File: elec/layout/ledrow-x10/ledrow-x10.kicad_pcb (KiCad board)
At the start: 2 copper layers, 20 parts

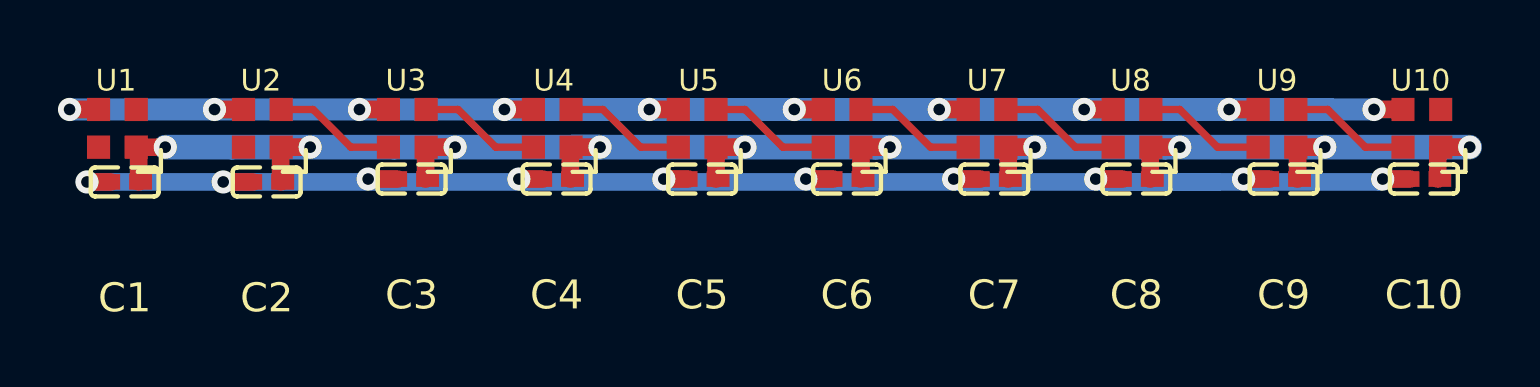
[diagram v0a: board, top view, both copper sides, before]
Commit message: fixing
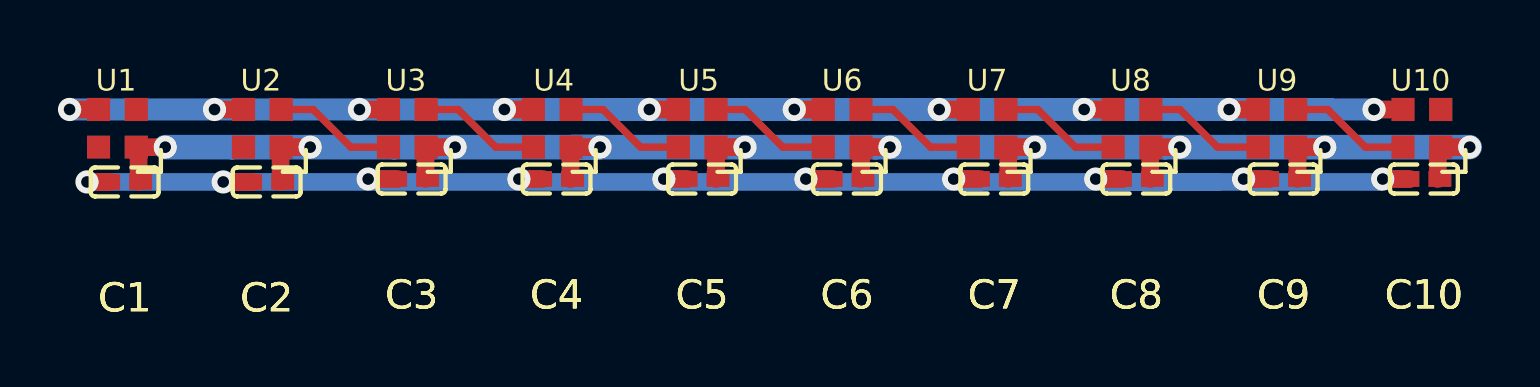
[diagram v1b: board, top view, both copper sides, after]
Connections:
- net vcc-4 renamed io-4
- U1 pad 2: vcc-2 -> io
- U10 pad 4: io -> vcc
- U2 pad 2: io-1 -> io-2
- U2 pad 4: vcc-2 -> io
- U3 pad 2: io-2 -> io-5
- U3 pad 4: io-1 -> io-2
- U4 pad 2: vcc-1 -> io-3
- U4 pad 4: io-2 -> io-5
- U5 pad 4: vcc-1 -> io-3
- U6 pad 2: vcc -> io-6
- U7 pad 2: vcc-3 -> io-1
- U7 pad 4: vcc -> io-6
- U8 pad 2: io-3 -> vcc-1
- U8 pad 4: vcc-3 -> io-1
- U9 pad 2: io -> vcc
- U9 pad 4: io-3 -> vcc-1
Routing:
- net vcc-3: track 4.24 -> 0.00 mm
- net io-6: track 0.00 -> 4.24 mm
- net io-5: track 0.00 -> 4.24 mm
- net io: track 4.24 -> 0.00 mm

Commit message: build with v3
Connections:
- U1 pad 2: io -> io-4
- U10 pad 4: vcc -> io-2
- U2 pad 2: io-2 -> io
- U2 pad 4: io -> io-4
- U3 pad 2: io-5 -> vcc
- U3 pad 4: io-2 -> io
- U4 pad 2: io-3 -> vcc-2
- U4 pad 4: io-5 -> vcc
- U5 pad 2: io-4 -> io-3
- U5 pad 4: io-3 -> vcc-2
- U6 pad 2: io-6 -> io-1
- U6 pad 4: io-4 -> io-3
- U7 pad 2: io-1 -> vcc-1
- U7 pad 4: io-6 -> io-1
- U8 pad 2: vcc-1 -> vcc-3
- U8 pad 4: io-1 -> vcc-1
- U9 pad 2: vcc -> io-2
- U9 pad 4: vcc-1 -> vcc-3
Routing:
- net vcc-2: track 0.00 -> 4.24 mm
- net io-6: track 4.24 -> 0.00 mm
- net io-5: track 4.24 -> 0.00 mm
- net io: track 0.00 -> 4.24 mm
- net vcc-3: track 0.00 -> 4.24 mm
- net io-4: track 4.24 -> 0.00 mm
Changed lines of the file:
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@@
     (net 1 "hv")
     (net 2 "gnd")
-    (net 3 "io-2")
-    (net 4 "io")
-    (net 5 "io-5")
-    (net 6 "io-3")
-    (net 7 "io-4")
-    (net 8 "io-6")
-    (net 9 "io-1")
-    (net 10 "vcc-1")
-    (net 11 "vcc")
+    (net 3 "io")
+    (net 4 "io-4")
+    (net 5 "vcc")
+    (net 6 "vcc-2")
+    (net 7 "io-3")
+    (net 8 "io-1")
+    (net 9 "vcc-1")
+    (net 10 "vcc-3")
+    (net 11 "io-2")
     (net 12 "DOUT")
     (net 13 "DIN")
@@
             (size 0.8 0.8)
             (layers "F.Cu" "F.Mask" "F.Paste")
-            (net 11 "vcc")
+            (net 11 "io-2")
             (pintype "stereo")
         )
@@
             (size 0.8 0.8)
             (layers "F.Cu" "F.Mask" "F.Paste")
-            (net 10 "vcc-1")
+            (net 10 "vcc-3")
             (pintype "stereo")
         )
@@
             (size 0.8 0.8)
             (layers "F.Cu" "F.Mask" "F.Paste")
-            (net 3 "io-2")
+            (net 3 "io")
             (pintype "stereo")
         )
@@
             (size 0.8 0.8)
             (layers "F.Cu" "F.Mask" "F.Paste")
-            (net 4 "io")
+            (net 4 "io-4")
             (pintype "stereo")
         )
@@
             (size 0.8 0.8)
             (layers "F.Cu" "F.Mask" "F.Paste")
-            (net 4 "io")
+            (net 4 "io-4")
             (pintype "stereo")
         )
@@
             (size 0.8 0.8)
             (layers "F.Cu" "F.Mask" "F.Paste")
-            (net 9 "io-1")
+            (net 9 "vcc-1")
             (pintype "stereo")
         )
@@
             (size 0.8 0.8)
             (layers "F.Cu" "F.Mask" "F.Paste")
-            (net 8 "io-6")
+            (net 8 "io-1")
             (pintype "stereo")
         )
@@
             (size 0.8 0.8)
             (layers "F.Cu" "F.Mask" "F.Paste")
-            (net 7 "io-4")
+            (net 7 "io-3")
             (pintype "stereo")
         )
@@
             (size 0.8 0.8)
             (layers "F.Cu" "F.Mask" "F.Paste")
-            (net 6 "io-3")
+            (net 6 "vcc-2")
             (pintype "stereo")
         )
@@
             (size 0.8 0.8)
             (layers "F.Cu" "F.Mask" "F.Paste")
-            (net 11 "vcc")
+            (net 11 "io-2")
             (pintype "stereo")
         )
@@
             (size 0.8 0.8)
             (layers "F.Cu" "F.Mask" "F.Paste")
-            (net 6 "io-3")
+            (net 6 "vcc-2")
             (pintype "stereo")
         )
@@
             (size 0.8 0.8)
             (layers "F.Cu" "F.Mask" "F.Paste")
-            (net 5 "io-5")
+            (net 5 "vcc")
             (pintype "stereo")
         )
@@
             (size 0.8 0.8)
             (layers "F.Cu" "F.Mask" "F.Paste")
-            (net 5 "io-5")
+            (net 5 "vcc")
             (pintype "stereo")
         )
@@
             (size 0.8 0.8)
             (layers "F.Cu" "F.Mask" "F.Paste")
-            (net 3 "io-2")
+            (net 3 "io")
             (pintype "stereo")
         )
@@
             (size 0.8 0.8)
             (layers "F.Cu" "F.Mask" "F.Paste")
-            (net 10 "vcc-1")
+            (net 10 "vcc-3")
             (pintype "stereo")
         )
@@
             (size 0.8 0.8)
             (layers "F.Cu" "F.Mask" "F.Paste")
-            (net 9 "io-1")
+            (net 9 "vcc-1")
             (pintype "stereo")
         )
@@
             (size 0.8 0.8)
             (layers "F.Cu" "F.Mask" "F.Paste")
-            (net 8 "io-6")
+            (net 8 "io-1")
             (pintype "stereo")
         )
@@
             (size 0.8 0.8)
             (layers "F.Cu" "F.Mask" "F.Paste")
-            (net 7 "io-4")
+            (net 7 "io-3")
             (pintype "stereo")
         )
